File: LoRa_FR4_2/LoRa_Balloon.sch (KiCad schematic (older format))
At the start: 63 parts, among them J2 Qwicc_6-pin, U1 SKY67013-396LF_CID141, U2 SX1272IMLTRICT-ND_CID104, U3 SKY67013-396LF_CID141, U4 PE4259_CID105, U5 ATMEGA328P-AU, U6 XCL205, X1 X1E0000210162_CID142, X2 7A-12.000MAAJ-T_CID117

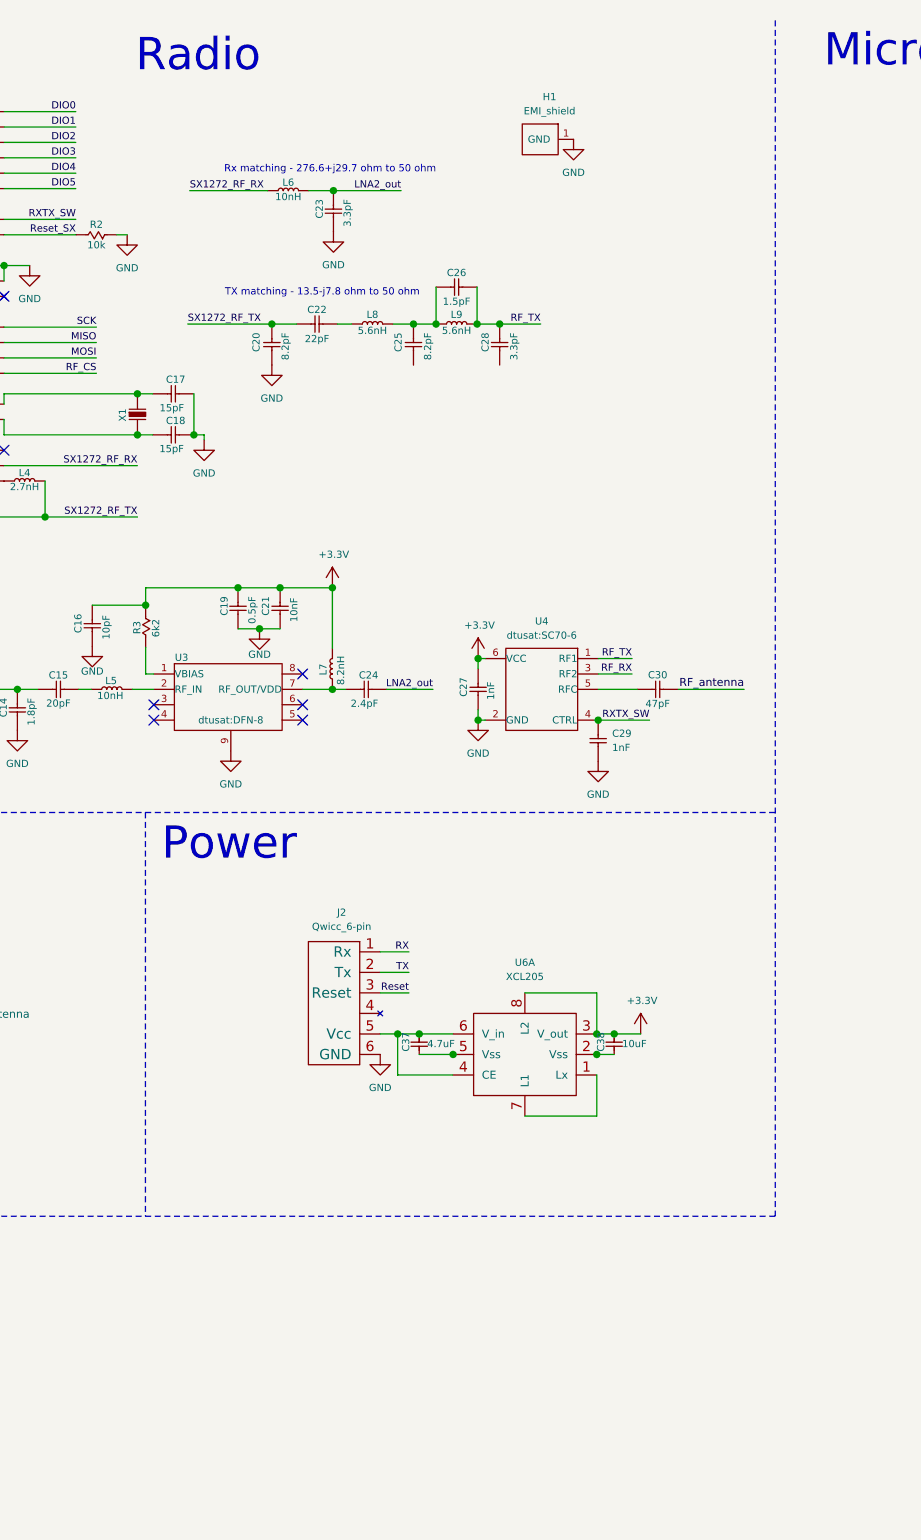
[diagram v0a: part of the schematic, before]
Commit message: New FR4 versions
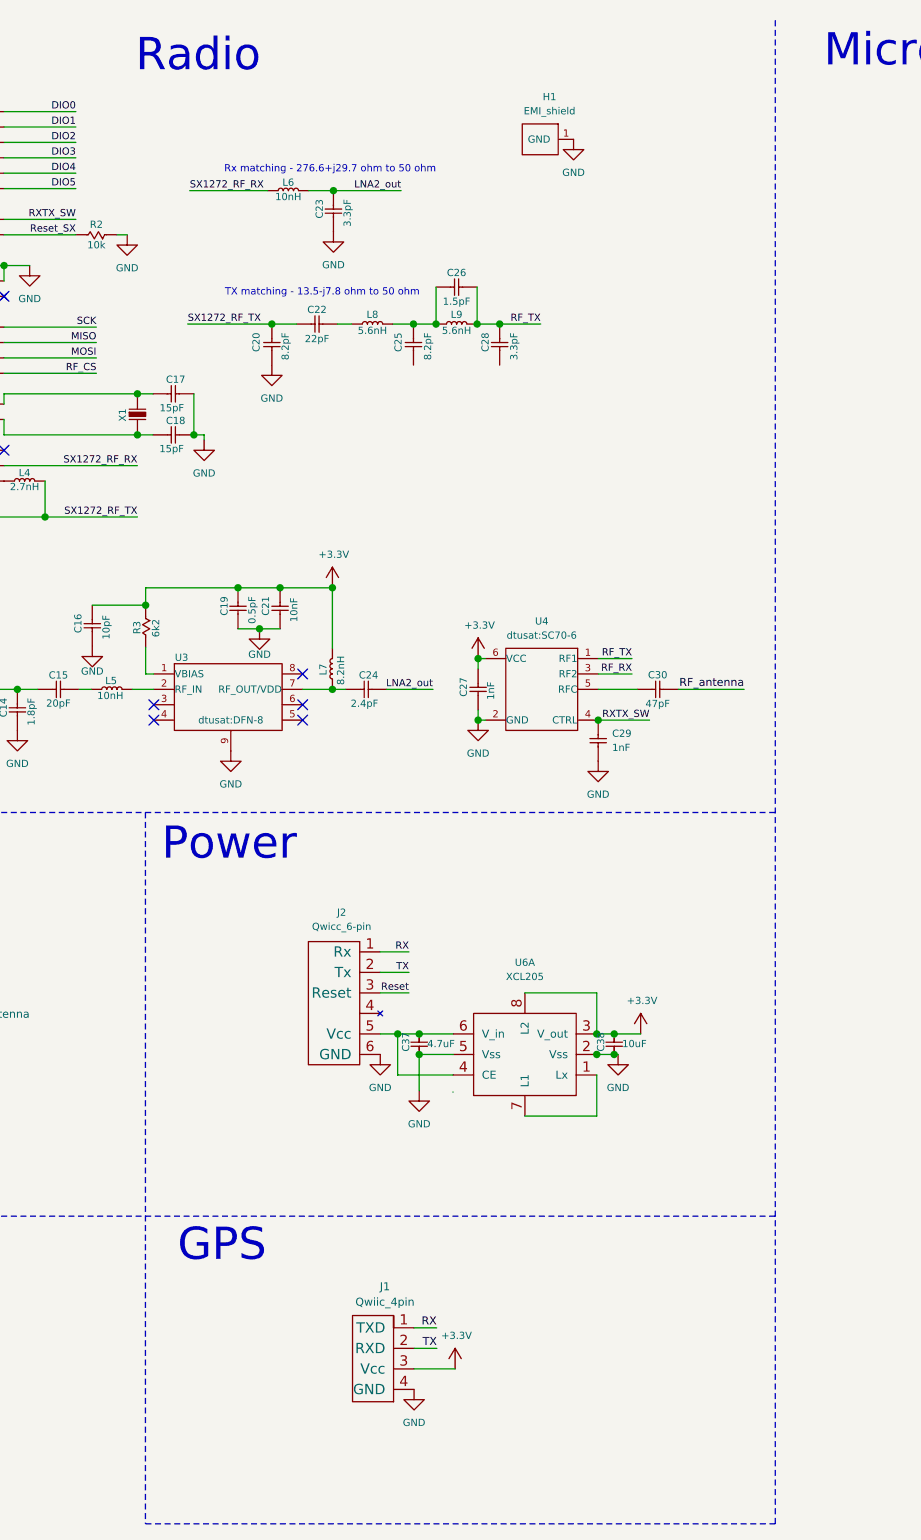
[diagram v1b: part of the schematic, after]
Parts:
- added J1: Qwiic_4pin, dtusat:Qwiic_4-pin, symbol connectors:Qwiic_4pin
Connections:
- wire segments 170 -> 175
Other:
- note added: "GPS\n"
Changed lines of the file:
@@
 Wire Wire Line
 	2542 1440 2892 1440
-$Comp
-L dtusat-ic:XCL205 U6
-U 1 1 5DF7C563
-P 5080 5459
-F 0 "U6" H 5080 5061 35  0000 C CNN
-F 1 "XCL205" H 5080 5130 35  0000 C CNN
-F 2 "dtusat:XCL205" H 5030 5009 35  0001 C CNN
-F 3 "" H 5030 5009 35  0001 C CNN
-	1    5080 5459
-	-1   0    0    1
-$EndComp
 Wire Wire Line
 	4375 5409 4460 5409
@@
 Wire Wire Line
 	4565 5409 4730 5409
-Wire Wire Line
-	4731 5509 4730 5509
-Connection ~ 4730 5509
-Wire Wire Line
-	4730 5509 4565 5509
 $Comp
 L dtusat-capacitors:C_1206_4.7uF_CID2013_small C38
@@
 $EndComp
 Wire Wire Line
-	5429 5509 5430 5509
-Connection ~ 5430 5509
-Wire Wire Line
-	5430 5509 5515 5509
-Wire Wire Line
 	5429 5409 5430 5409
 Connection ~ 5430 5409
@@
 	1534 5342 1894 5342
 Wire Notes Line
-	6300 470  6300 6297
-Wire Notes Line
 	470  4330 6300 4330
-Wire Notes Line
-	3231 4329 3231 6297
 Wire Notes Line
 	470  6297 6300 6297
@@
 Text Notes 8153 714  2    157  ~ 0
 Microcontroller
+$Comp
+L dtusat-power:GND #PWR031
+U 1 1 5E0DCCF1
+P 4565 5686
+F 0 "#PWR031" H 4565 5436 35  0001 C CNN
+F 1 "GND" H 4565 5524 35  0000 C CNN
+F 2 "" H 4565 5686 35  0000 C CNN
+F 3 "" H 4565 5686 35  0000 C CNN
+	1    4565 5686
+	1    0    0    -1
+$EndComp
+Wire Wire Line
+	4730 5692 4729 5692
+Wire Wire Line
+	5429 5509 5430 5509
+Wire Wire Line
+	5430 5509 5515 5509
+Connection ~ 5430 5509
+$Comp
+L dtusat-ic:XCL205 U6
+U 1 1 5DF7C563
+P 5080 5459
+F 0 "U6" H 5080 5061 35  0000 C CNN
+F 1 "XCL205" H 5080 5130 35  0000 C CNN
+F 2 "dtusat:XCL205" H 5030 5009 35  0001 C CNN
+F 3 "" H 5030 5009 35  0001 C CNN
+	1    5080 5459
+	-1   0    0    1
+$EndComp
+Wire Wire Line
+	4565 5509 4730 5509
+Wire Wire Line
+	4565 5509 4565 5686
+Connection ~ 4565 5509
+$Comp
+L dtusat-power:GND #PWR039
+U 1 1 5E108C7C
+P 5534 5509
+F 0 "#PWR039" H 5534 5259 35  0001 C CNN
+F 1 "GND" H 5534 5347 35  0000 C CNN
+F 2 "" H 5534 5509 35  0000 C CNN
+F 3 "" H 5534 5509 35  0000 C CNN
+	1    5534 5509
+	1    0    0    -1
+$EndComp
+Wire Wire Line
+	5515 5509 5534 5509
+Connection ~ 5515 5509
+$Comp
+L connectors:Qwiic_4pin J1
+U 1 1 5DFAC160
+P 4400 6981
+F 0 "J1" H 4398 7322 39  0000 C CNN
+F 1 "Qwiic_4pin" H 4398 7247 39  0000 C CNN
+F 2 "dtusat:Qwiic_4-pin" H 4400 6921 39  0001 C CNN
+F 3 "" H 4400 6921 39  0001 C CNN
+	1    4400 6981
+	1    0    0    -1
+$EndComp
+Wire Wire Line
+	4540 6841 4650 6841
+Wire Wire Line
+	4540 6941 4651 6941
+Text Label 4650 6841 2    39   ~ 0
+RX
+Text Label 4651 6941 2    39   ~ 0
+TX
+$Comp
+L dtusat-power:GND #PWR025
+U 1 1 5DFC2C64
+P 4540 7141
+F 0 "#PWR025" H 4540 6891 35  0001 C CNN
+F 1 "GND" H 4540 6979 35  0000 C CNN
+F 2 "" H 4540 7141 35  0000 C CNN
+F 3 "" H 4540 7141 35  0000 C CNN
+	1    4540 7141
+	1    0    0    -1
+$EndComp
+$Comp
+L dtusat-power:+3.3V #PWR038
+U 1 1 5DFC3EDD
+P 4740 7041
+F 0 "#PWR038" H 4740 6891 35  0001 C CNN
+F 1 "+3.3V" H 4747 7203 35  0000 C CNN
+F 2 "" H 4740 7041 35  0000 C CNN
+F 3 "" H 4740 7041 35  0000 C CNN
+	1    4740 7041
+	1    0    0    -1
+$EndComp
+Wire Wire Line
+	4540 7041 4740 7041
+Wire Notes Line
+	3231 7796 6300 7796
+Wire Notes Line
+	6300 470  6300 7796
+Wire Notes Line
+	3231 4329 3231 7796
+Text Notes 3821 6534 2    157  ~ 0
+GPS\n
 $EndSCHEMATC
